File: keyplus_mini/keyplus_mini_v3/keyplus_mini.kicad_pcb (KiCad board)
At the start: 2 copper layers, 24.1 x 23 mm, 23 parts, among them J1 USB_C_Receptacle, J2 Conn_02x09_Odd_Even, J3 CONN_01X01, J4 Conn_02x09_Odd_Even, U1 MCP1700-3302E_SOT23, U2 ATXMEGA-A4U-EPAD

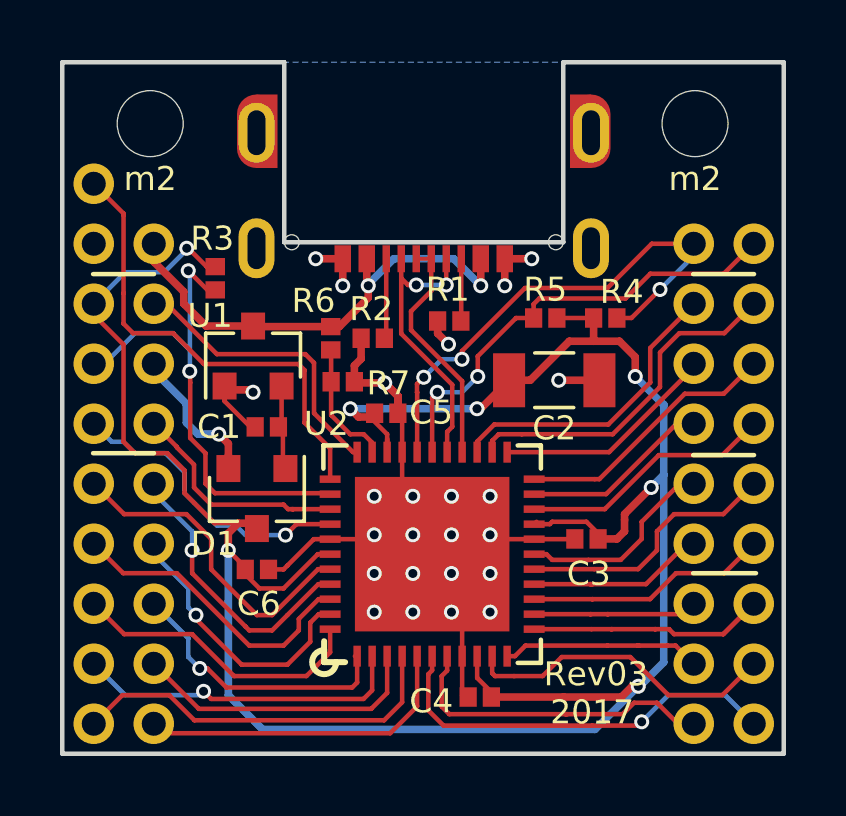
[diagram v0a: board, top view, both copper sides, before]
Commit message: cleanup keyplus mini_v3
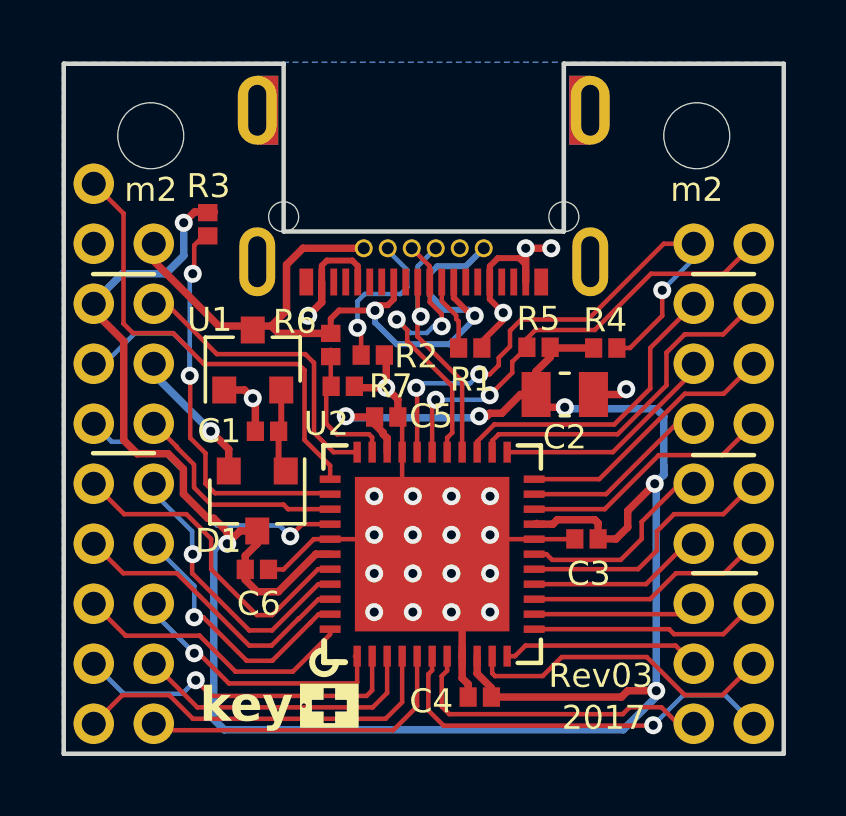
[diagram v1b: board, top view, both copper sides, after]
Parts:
- removed OSHW_Logo: G***, logo:OSHW_3x3mm_SilkS
- added ?: REF**, logo:key+_5mm, F.Cu at (203.2, 114.5)
- added ?: , logo:OSHW_3x3mm_SilkS, B.Cu at (207.1, 112.4)
- C2: footprint Capacitor_SMD:C_1206_3216Metric -> Capacitor_SMD:C_0805_2012Metric
- J1: footprint conn_usb:USB_TypeC_239FC14-00276T-H -> conn_usb:USB_TypeC_Hirose_CX70M-24P1
- moved R3 1.82 mm to (200.8, 98.3)
- moved R1 1.14 mm to (209.6, 102.5), turned to 0 degrees
- moved R5 1.00 mm to (211.8, 102.5)
- moved J1 1.00 mm to (208.0, 92.0)
- moved R4 1.00 mm to (214.1, 102.5)
- moved C2 0.59 mm to (212.7, 104.0)
- moved R2 0.56 mm to (206.3, 102.7), turned to 0 degrees
- moved ? 0.41 mm to (217.1, 95.4)
- moved ? 0.40 mm to (198.9, 95.4)
- moved R6 0.22 mm to (204.9, 102.4)
- moved R7 0.15 mm to (205.3, 103.8)
- moved C1 0.14 mm to (202.8, 105.2)
- moved U1 0.13 mm to (202.3, 102.9)
- moved C5 0.12 mm to (206.8, 104.8)
- moved D1 0.08 mm to (202.4, 107.6)
- renumbered REF** to ?
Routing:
- net +5V: track 16.7 -> 27.3 mm
- net GND: track 25.2 -> 30.4 mm, vias 24 -> 23
- net +3V3: track 82.2 -> 86.3 mm
- net Net-(J1-PadB5): track 2.68 -> 5.51 mm, vias 0 -> 1
- net /PCL: track 16.8 -> 18.6 mm
- net /PE1: track 17.5 -> 19.1 mm
- net /PC2: track 9.31 -> 7.81 mm
- net /D-: track 7.93 -> 9.04 mm, vias 0 -> 1
- net /PA5: track 9.44 -> 10.2 mm
- net Net-(R6-Pad2): track 4.24 -> 4.94 mm
- net /PE0: track 15.6 -> 15.0 mm
- net Net-(C1-Pad2): track 2.61 -> 3.13 mm
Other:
- board size 24.1 x 23 mm -> 24 x 23 mm
- net class 5v removed
- net class Default: via_dia 0.5 -> 0.6
- net class Power added: clearance 0.1524, trace_width 0.25, via_dia 0.6, via_drill 0.3
- net class temp: via_dia 0.5 -> 0.6
- rule trace_min: 0.127 -> 0.1524
- rule via_min_drill: 0.2032 -> 0.3
- rule via_min_size: 0.4572 -> 0.6
- board text added: "keyplus mini"
- board text added: "©jem"
- board text removed: "SPI"
